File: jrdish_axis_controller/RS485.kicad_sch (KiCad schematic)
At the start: 46 parts, among them CN3 KF2EDGR-2.54-4P, CN4 KF2EDGR-2.54-4P, CN5 KF2EDGR-2.54-4P, U2 ISOW1432BDFMR, U3 ISOW1432BDFMR

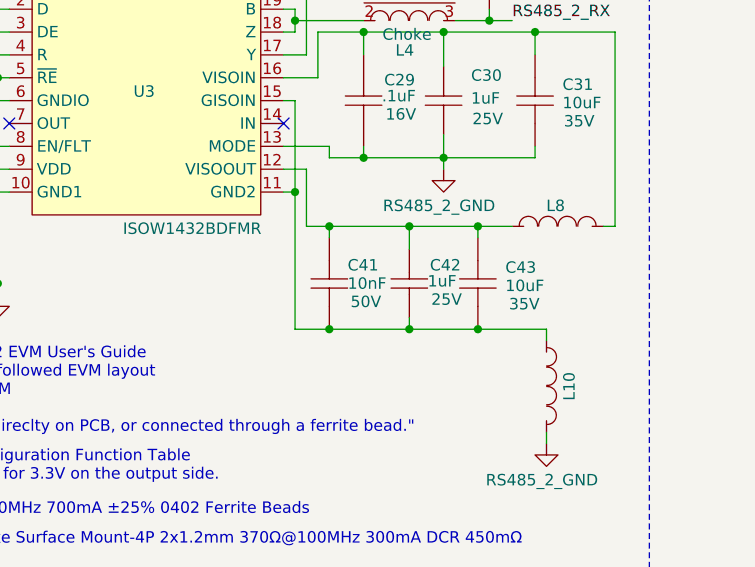
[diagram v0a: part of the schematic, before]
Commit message: Layout complete
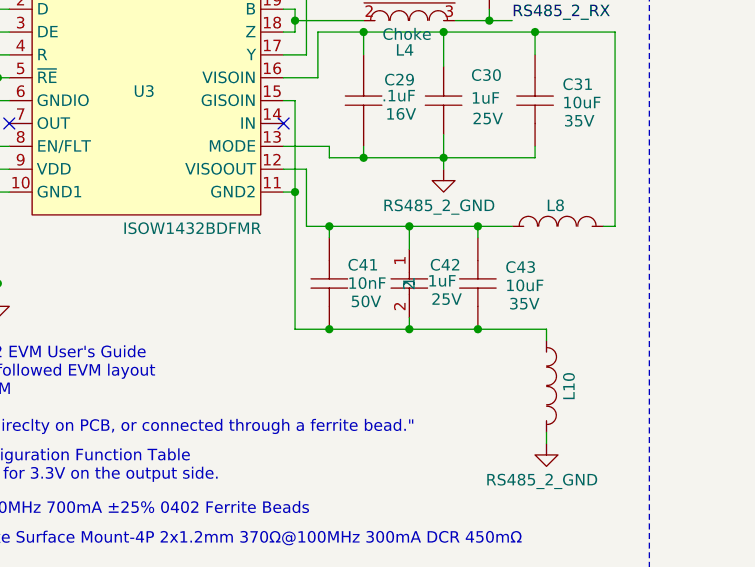
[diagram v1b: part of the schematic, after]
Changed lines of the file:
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@@
 	)
 	(symbol
+		(lib_name "CL10A105KA8NNNC_7")
 		(lib_id "MyParts:CL10A105KA8NNNC")
 		(at 255.27 58.42 270)
@@
 			)
 		)
-		(property "Datasheet" "https://www.lcsc.com/datasheet/C5673.pdf?spm=wm.sxq.inf.ggs___wm.ssy.bg.0.cbh&lcsc_vid=FFBaV1wHQFldUVICFgBfBVJTQVJWXgBfEQRYBAFQE1YxVlNRQFNXUV1UR1laVDsOAxUeFF5JWBYZEEoKFBINSQcJGk4dAgUUFAk%3D"
+		(property "Datasheet" "https://lcsc.com/product-detail/Multilayer-Ceramic-Capacitors-MLCC-SMD-SMT_SAMSUNG_CL10A105KA8NNNC_1uF-105-10-25V_C5673.html"
 			(at 245.11 58.42 0)
 			(hide yes)
@@
 	)
 	(symbol
+		(lib_name "CL10A105KA8NNNC_5")
 		(lib_id "MyParts:CL10A105KA8NNNC")
 		(at 175.26 52.07 270)
@@
 			)
 		)
-		(property "Datasheet" "https://www.lcsc.com/datasheet/C5673.pdf?spm=wm.sxq.inf.ggs___wm.ssy.bg.0.cbh&lcsc_vid=FFBaV1wHQFldUVICFgBfBVJTQVJWXgBfEQRYBAFQE1YxVlNRQFNXUV1UR1laVDsOAxUeFF5JWBYZEEoKFBINSQcJGk4dAgUUFAk%3D"
+		(property "Datasheet" "https://lcsc.com/product-detail/Multilayer-Ceramic-Capacitors-MLCC-SMD-SMT_SAMSUNG_CL10A105KA8NNNC_1uF-105-10-25V_C5673.html"
 			(at 165.1 52.07 0)
 			(hide yes)
@@
 	)
 	(symbol
+		(lib_name "CL10A105KA8NNNC_3")
 		(lib_id "MyParts:CL10A105KA8NNNC")
 		(at 39.37 52.07 270)
@@
 			)
 		)
-		(property "Datasheet" "https://www.lcsc.com/datasheet/C5673.pdf?spm=wm.sxq.inf.ggs___wm.ssy.bg.0.cbh&lcsc_vid=FFBaV1wHQFldUVICFgBfBVJTQVJWXgBfEQRYBAFQE1YxVlNRQFNXUV1UR1laVDsOAxUeFF5JWBYZEEoKFBINSQcJGk4dAgUUFAk%3D"
+		(property "Datasheet" "https://lcsc.com/product-detail/Multilayer-Ceramic-Capacitors-MLCC-SMD-SMT_SAMSUNG_CL10A105KA8NNNC_1uF-105-10-25V_C5673.html"
 			(at 29.21 52.07 0)
 			(hide yes)
@@
 	)
 	(symbol
+		(lib_name "CL10A105KA8NNNC_2")
 		(lib_id "MyParts:CL10A105KA8NNNC")
 		(at 115.57 78.74 270)
@@
 			)
 		)
-		(property "Datasheet" "https://www.lcsc.com/datasheet/C5673.pdf?spm=wm.sxq.inf.ggs___wm.ssy.bg.0.cbh&lcsc_vid=FFBaV1wHQFldUVICFgBfBVJTQVJWXgBfEQRYBAFQE1YxVlNRQFNXUV1UR1laVDsOAxUeFF5JWBYZEEoKFBINSQcJGk4dAgUUFAk%3D"
+		(property "Datasheet" "https://lcsc.com/product-detail/Multilayer-Ceramic-Capacitors-MLCC-SMD-SMT_SAMSUNG_CL10A105KA8NNNC_1uF-105-10-25V_C5673.html"
 			(at 105.41 78.74 0)
 			(hide yes)
@@
 	)
 	(symbol
+		(lib_name "CL10A105KA8NNNC_1")
 		(lib_id "MyParts:CL10A105KA8NNNC")
 		(at 119.38 58.42 270)
@@
 			)
 		)
-		(property "Datasheet" "https://www.lcsc.com/datasheet/C5673.pdf?spm=wm.sxq.inf.ggs___wm.ssy.bg.0.cbh&lcsc_vid=FFBaV1wHQFldUVICFgBfBVJTQVJWXgBfEQRYBAFQE1YxVlNRQFNXUV1UR1laVDsOAxUeFF5JWBYZEEoKFBINSQcJGk4dAgUUFAk%3D"
+		(property "Datasheet" "https://lcsc.com/product-detail/Multilayer-Ceramic-Capacitors-MLCC-SMD-SMT_SAMSUNG_CL10A105KA8NNNC_1uF-105-10-25V_C5673.html"
 			(at 109.22 58.42 0)
 			(hide yes)
@@
 	)
 	(symbol
+		(lib_name "CL10A105KA8NNNC_4")
 		(lib_id "MyParts:CL10A105KA8NNNC")
 		(at 52.07 72.39 270)
@@
 			)
 		)
-		(property "Datasheet" "https://www.lcsc.com/datasheet/C5673.pdf?spm=wm.sxq.inf.ggs___wm.ssy.bg.0.cbh&lcsc_vid=FFBaV1wHQFldUVICFgBfBVJTQVJWXgBfEQRYBAFQE1YxVlNRQFNXUV1UR1laVDsOAxUeFF5JWBYZEEoKFBINSQcJGk4dAgUUFAk%3D"
+		(property "Datasheet" "https://lcsc.com/product-detail/Multilayer-Ceramic-Capacitors-MLCC-SMD-SMT_SAMSUNG_CL10A105KA8NNNC_1uF-105-10-25V_C5673.html"
 			(at 41.91 72.39 0)
 			(hide yes)
@@
 	)
 	(symbol
+		(lib_name "CL10A105KA8NNNC_6")
 		(lib_id "MyParts:CL10A105KA8NNNC")
 		(at 187.96 72.39 270)
@@
 			)
 		)
-		(property "Datasheet" "https://www.lcsc.com/datasheet/C5673.pdf?spm=wm.sxq.inf.ggs___wm.ssy.bg.0.cbh&lcsc_vid=FFBaV1wHQFldUVICFgBfBVJTQVJWXgBfEQRYBAFQE1YxVlNRQFNXUV1UR1laVDsOAxUeFF5JWBYZEEoKFBINSQcJGk4dAgUUFAk%3D"
+		(property "Datasheet" "https://lcsc.com/product-detail/Multilayer-Ceramic-Capacitors-MLCC-SMD-SMT_SAMSUNG_CL10A105KA8NNNC_1uF-105-10-25V_C5673.html"
 			(at 177.8 72.39 0)
 			(hide yes)
@@
 			)
 		)
-		(property "Datasheet" "https://www.lcsc.com/datasheet/C5673.pdf?spm=wm.sxq.inf.ggs___wm.ssy.bg.0.cbh&lcsc_vid=FFBaV1wHQFldUVICFgBfBVJTQVJWXgBfEQRYBAFQE1YxVlNRQFNXUV1UR1laVDsOAxUeFF5JWBYZEEoKFBINSQcJGk4dAgUUFAk%3D"
+		(property "Datasheet" "https://lcsc.com/product-detail/Multilayer-Ceramic-Capacitors-MLCC-SMD-SMT_SAMSUNG_CL10A105KA8NNNC_1uF-105-10-25V_C5673.html"
 			(at 241.3 78.74 0)
 			(hide yes)
